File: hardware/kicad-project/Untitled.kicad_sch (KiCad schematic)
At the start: 42 parts, among them CN2 ST-0322D00-071-1A2H, Q1 DMG2301L-7, SW10 TS-1187A-B-A-B, SW9 TS-1187A-B-A-B, U1 ESP32-S3-WROOM-1(N8R2), U2 MCP73831-2ACI/MC, U3 ME6217C33P5G, U6 MAX98357AETE+T

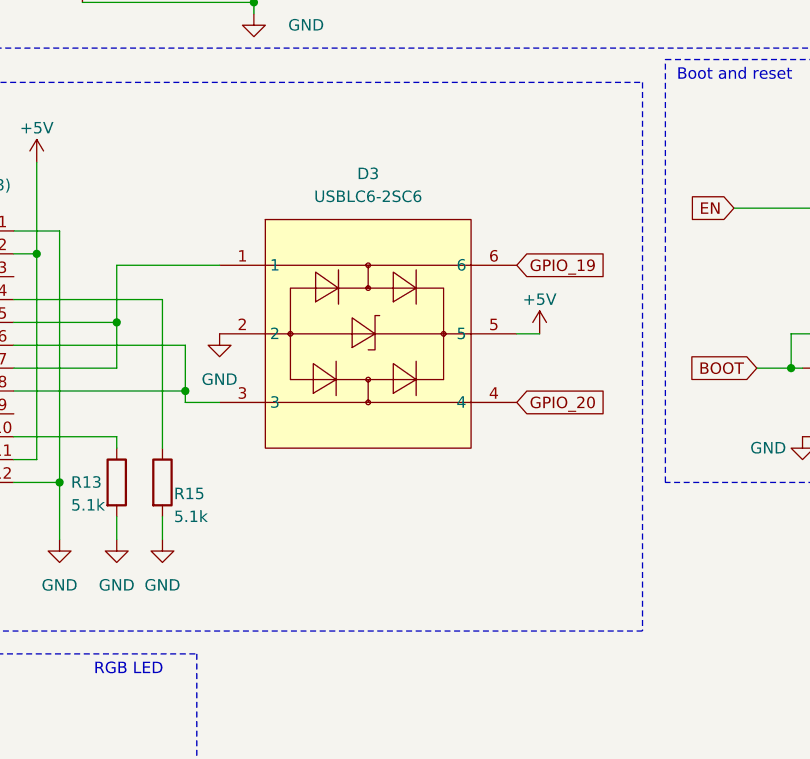
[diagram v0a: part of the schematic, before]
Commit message: rev2
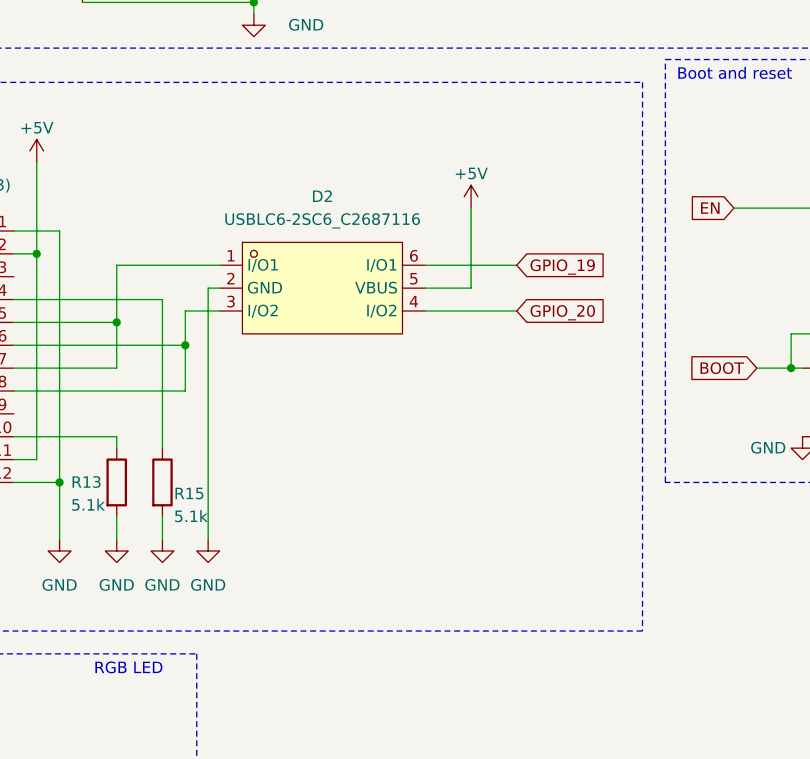
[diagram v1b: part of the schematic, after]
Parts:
- removed D3: USBLC6-2SC6, easyeda2kicad:SOT-23-6_L2.9-W1.6-P0.95-LS2.8-BL, symbol easyedaToKicad:USBLC6-2SC6
- added D2: USBLC6-2SC6_C2687116, easyeda2kicad:SOT-23-6_L2.9-W1.6-P0.95-LS2.8-BL, symbol easyedaToKicad:USBLC6-2SC6_C2687116
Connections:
- net +5V: now also D2.5 (VBUS)
- net GND: now also D2.2 (GND)
- net GPIO_19: now also D2.6 (I/O1)
- net GPIO_20: now also D2.4 (I/O2)
- net at USB1.5 (DN2), USB1.7 (DN1): now also D2.1 (I/O1)
- net at USB1.6 (DP1), USB1.8 (DP2): now also D2.3 (I/O2)
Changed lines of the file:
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@@
   (junction (at 104.14 152.4) (diameter 0) (color 0 0 0 0)
   )
+  (junction (at 166.37 123.19) (diameter 0) (color 0 0 0 0)
+  )
   (junction (at 44.45 171.45) (diameter 0) (color 0 0 0 0)
   )
@@
   (junction (at 104.14 45.72) (diameter 0) (color 0 0 0 0)
   )
-  (junction (at 166.37 128.27) (diameter 0) (color 0 0 0 0)
-  )
   (no_connect (at 50.8 91.44))
   (no_connect (at 48.26 91.44))
@@
     (stroke (width 0) (type default))
   )
-  (wire (pts (xy 166.37 129.54) (xy 170.18 129.54))
-    (stroke (width 0) (type default))
-  )
   (wire (pts (xy 63.5 91.44) (xy 63.5 95.25))
     (stroke (width 0) (type default))
@@
     (stroke (width 0) (type default))
   )
-  (wire (pts (xy 205.74 121.92) (xy 203.2 121.92))
-    (stroke (width 0) (type default))
-  )
   (wire (pts (xy 227.33 64.77) (xy 227.33 80.01))
     (stroke (width 0) (type default))
@@
     (stroke (width 0) (type default))
   )
+  (wire (pts (xy 168.91 116.84) (xy 168.91 144.78))
+    (stroke (width 0) (type default))
+  )
   (wire (pts (xy 158.75 125.73) (xy 158.75 120.65))
     (stroke (width 0) (type default))
   )
+  (wire (pts (xy 193.04 119.38) (xy 203.2 119.38))
+    (stroke (width 0) (type default))
+  )
   (wire (pts (xy 36.83 179.07) (xy 36.83 193.04))
     (stroke (width 0) (type default))
@@
     (stroke (width 0) (type default))
   )
+  (wire (pts (xy 170.18 116.84) (xy 168.91 116.84))
+    (stroke (width 0) (type default))
+  )
   (wire (pts (xy 97.79 29.21) (xy 102.87 29.21))
     (stroke (width 0) (type default))
@@
     (stroke (width 0) (type default))
   )
+  (wire (pts (xy 198.12 107.95) (xy 198.12 116.84))
+    (stroke (width 0) (type default))
+  )
   (wire (pts (xy 149.86 102.87) (xy 149.86 113.03))
     (stroke (width 0) (type default))
@@
     (stroke (width 0) (type default))
   )
+  (wire (pts (xy 193.04 114.3) (xy 203.2 114.3))
+    (stroke (width 0) (type default))
+  )
   (wire (pts (xy 233.68 125.73) (xy 234.95 125.73))
     (stroke (width 0) (type default))
@@
     (stroke (width 0) (type default))
   )
+  (wire (pts (xy 170.18 119.38) (xy 166.37 119.38))
+    (stroke (width 0) (type default))
+  )
   (wire (pts (xy 149.86 135.89) (xy 149.86 113.03))
     (stroke (width 0) (type default))
@@
     (stroke (width 0) (type default))
   )
-  (wire (pts (xy 166.37 128.27) (xy 166.37 129.54))
-    (stroke (width 0) (type default))
-  )
   (wire (pts (xy 87.63 60.96) (xy 83.82 60.96))
     (stroke (width 0) (type default))
@@
     (stroke (width 0) (type default))
   )
+  (wire (pts (xy 193.04 116.84) (xy 198.12 116.84))
+    (stroke (width 0) (type default))
+  )
   (wire (pts (xy 68.58 91.44) (xy 68.58 95.25))
     (stroke (width 0) (type default))
@@
     (stroke (width 0) (type default))
   )
+  (wire (pts (xy 166.37 119.38) (xy 166.37 123.19))
+    (stroke (width 0) (type default))
+  )
   (wire (pts (xy 92.71 124.46) (xy 92.71 147.32))
     (stroke (width 0) (type default))
@@
     )
   )
-  (global_label "GPIO_20" (shape input) (at 203.2 129.54 0) (fields_autoplaced)
+  (global_label "GPIO_20" (shape input) (at 203.2 119.38 0) (fields_autoplaced)
     (effects (font (size 1.27 1.27)) (justify left))
-    (property "Intersheetrefs" "${INTERSHEET_REFS}" (at 214.0471 129.54 0)
+    (property "Intersheetrefs" "${INTERSHEET_REFS}" (at 214.0471 119.38 0)
       (effects (font (size 1.27 1.27)) (justify left) hide)
     )
@@
     )
   )
-  (symbol (lib_id "power:+5V") (at 205.74 121.92 0) (unit 1)
+  (symbol (lib_id "power:+5V") (at 198.12 107.95 0) (unit 1)
     (in_bom yes) (on_board yes) (dnp no)
-    (property "Reference" "#PWR033" (at 205.74 125.73 0)
+    (property "Reference" "#PWR033" (at 198.12 111.76 0)
       (effects (font (size 1.27 1.27)) hide)
     )
-    (property "Value" "+5V" (at 205.74 118.11 0)
+    (property "Value" "+5V" (at 198.12 104.14 0)
       (effects (font (size 1.27 1.27)))
     )
-    (property "Footprint" "" (at 205.74 121.92 0)
+    (property "Footprint" "" (at 198.12 107.95 0)
       (effects (font (size 1.27 1.27)) hide)
     )
-    (property "Datasheet" "" (at 205.74 121.92 0)
+    (property "Datasheet" "" (at 198.12 107.95 0)
       (effects (font (size 1.27 1.27)) hide)
     )
@@
     )
   )
-  (symbol (lib_id "easyedaToKicad:USBLC6-2SC6") (at 186.69 121.92 0) (unit 1)
-    (in_bom yes) (on_board yes) (dnp no) (fields_autoplaced)
-    (property "Reference" "D3" (at 186.69 104.14 0)
-      (effects (font (size 1.27 1.27)))
-    )
-    (property "Value" "USBLC6-2SC6" (at 186.69 106.68 0)
-      (effects (font (size 1.27 1.27)))
-    )
-    (property "Footprint" "easyeda2kicad:SOT-23-6_L2.9-W1.6-P0.95-LS2.8-BL" (at 186.69 137.16 0)
-      (effects (font (size 1.27 1.27)) hide)
-    )
-    (property "Datasheet" "https://lcsc.com/product-detail/Diodes-ESD_STMicroelectronics_USBLC6-2SC6_USBLC6-2SC6_C7519.html" (at 186.69 139.7 0)
-      (effects (font (size 1.27 1.27)) hide)
-    )
-    (property "LCSC Part" "C7519" (at 186.69 142.24 0)
-      (effects (font (size 1.27 1.27)) hide)
-    )
-    (pin "1")
-    (pin "2")
-    (pin "3")
-    (pin "4")
-    (pin "5")
-    (pin "6")
-    (instances
-      (project "Untitled"
-        (path "/0de5ae84-7f75-4a5a-83a1-35d27fd1d8d2"
-          (reference "D3") (unit 1)
-        )
-      )
-    )
-  )
   (symbol (lib_id "Device:C") (at 97.79 25.4 180) (unit 1)
     (in_bom yes) (on_board yes) (dnp no)
@@
     )
   )
+  (symbol (lib_id "easyedaToKicad:USBLC6-2SC6_C2687116") (at 181.61 116.84 0) (unit 1)
+    (in_bom yes) (on_board yes) (dnp no) (fields_autoplaced)
+    (property "Reference" "D2" (at 181.61 106.68 0)
+      (effects (font (size 1.27 1.27)))
+    )
+    (property "Value" "USBLC6-2SC6_C2687116" (at 181.61 109.22 0)
+      (effects (font (size 1.27 1.27)))
+    )
+    (property "Footprint" "easyeda2kicad:SOT-23-6_L2.9-W1.6-P0.95-LS2.8-BL" (at 181.61 127 0)
+      (effects (font (size 1.27 1.27)) hide)
+    )
+    (property "Datasheet" "" (at 181.61 116.84 0)
+      (effects (font (size 1.27 1.27)) hide)
+    )
+    (property "LCSC Part" "C2687116" (at 181.61 129.54 0)
+      (effects (font (size 1.27 1.27)) hide)
+    )
+    (pin "1")
+    (pin "2")
+    (pin "3")
+    (pin "4")
+    (pin "5")
+    (pin "6")
+    (instances
+      (project "Untitled"
+        (path "/0de5ae84-7f75-4a5a-83a1-35d27fd1d8d2"
+          (reference "D2") (unit 1)
+        )
+      )
+    )
+  )
   (symbol (lib_id "Device:C") (at 252.73 111.76 0) (unit 1)
     (in_bom yes) (on_board yes) (dnp no)
@@
     )
   )
-  (symbol (lib_id "power:GND") (at 170.18 121.92 0) (unit 1)
+  (symbol (lib_id "power:GND") (at 168.91 144.78 0) (unit 1)
     (in_bom yes) (on_board yes) (dnp no) (fields_autoplaced)
-    (property "Reference" "#PWR038" (at 170.18 128.27 0)
+    (property "Reference" "#PWR038" (at 168.91 151.13 0)
       (effects (font (size 1.27 1.27)) hide)
     )
-    (property "Value" "GND" (at 170.18 127 0)
+    (property "Value" "GND" (at 168.91 149.86 0)
       (effects (font (size 1.27 1.27)))
     )
-    (property "Footprint" "" (at 170.18 121.92 0)
+    (property "Footprint" "" (at 168.91 144.78 0)
       (effects (font (size 1.27 1.27)) hide)
     )
-    (property "Datasheet" "" (at 170.18 121.92 0)
+    (property "Datasheet" "" (at 168.91 144.78 0)
       (effects (font (size 1.27 1.27)) hide)
     )
